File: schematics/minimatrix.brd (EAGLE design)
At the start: 32 x 32 mm, 10 parts

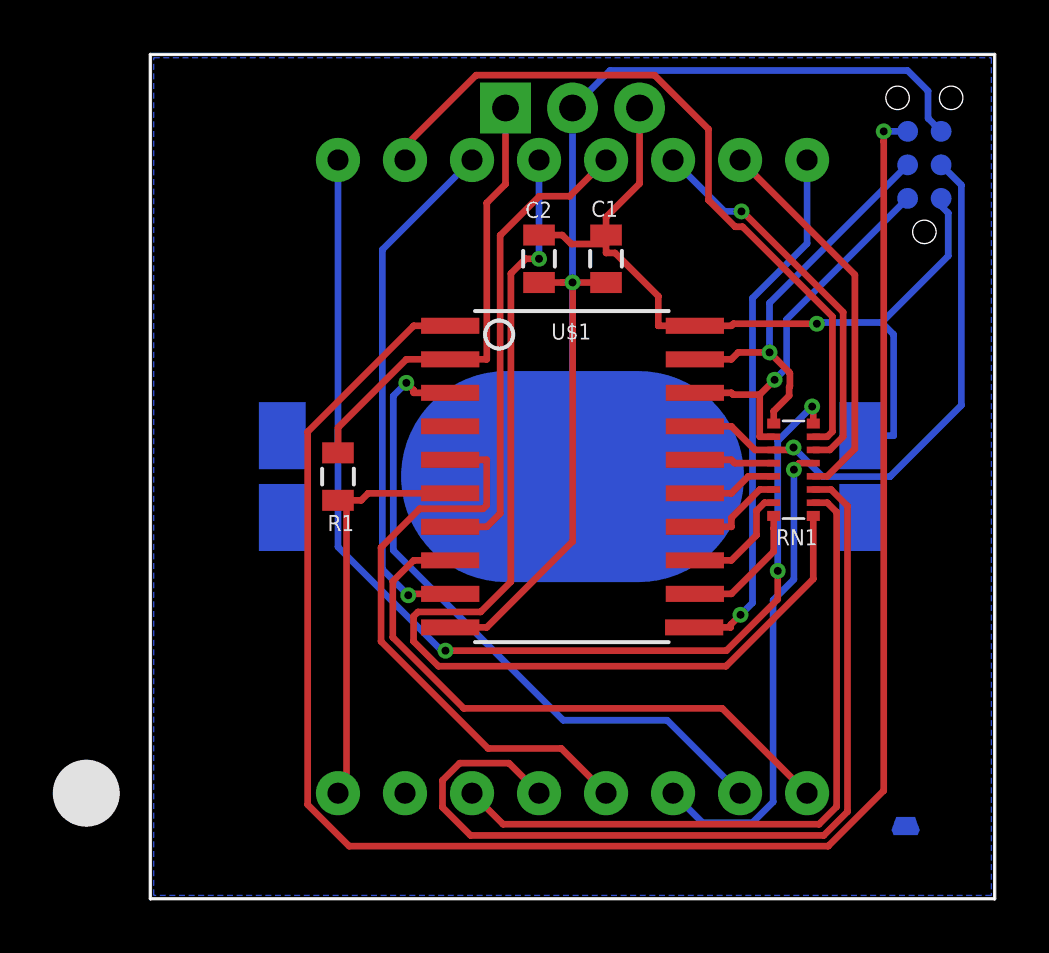
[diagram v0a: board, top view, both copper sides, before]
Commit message: ?
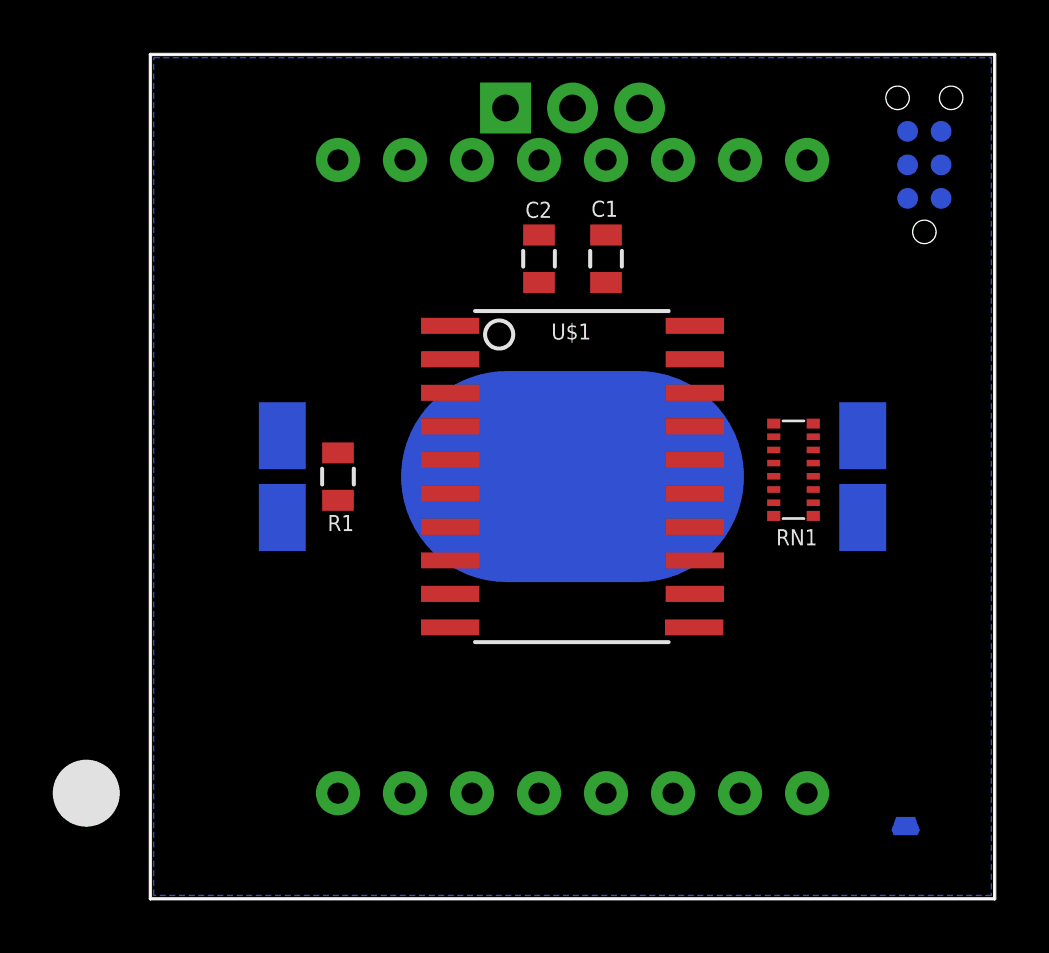
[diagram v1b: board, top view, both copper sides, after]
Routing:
- net N$2: track 70.4 -> 0.00 mm, vias 1 -> 0
- net GND: track 48.4 -> 0.00 mm, vias 1 -> 0
- net N$9: track 42.3 -> 0.00 mm, vias 3 -> 0
- net N$10: track 41.2 -> 0.00 mm, vias 1 -> 0
- net N$4: track 34.7 -> 0.00 mm
- net VCC: track 32.7 -> 0.00 mm, vias 1 -> 0
- net N$8: track 28.4 -> 0.00 mm
- net N$3: track 26.8 -> 0.00 mm
- net R6: track 25.4 -> 0.00 mm, vias 1 -> 0
- net R3: track 22.8 -> 0.00 mm
- net R8: track 22.2 -> 0.00 mm
- net C6: track 21.5 -> 0.00 mm, vias 1 -> 0
- net ROW1: track 20.3 -> 0.00 mm, vias 1 -> 0
- net R2: track 19.9 -> 0.00 mm, vias 1 -> 0
- net N$6: track 18.4 -> 0.00 mm, vias 1 -> 0
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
